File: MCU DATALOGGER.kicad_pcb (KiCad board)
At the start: 2 copper layers, 54.3 x 31.6 mm, 30 parts, among them J1 Conn_01x04_Pin, J2 Conn_01x04_Pin, J3 Conn_01x09_Pin, J4 Conn_02x03_Odd_Even, U1 24LC1025, U2 24LC1025, U4 ATMEGA328P-AU, U5 DS1337S_, Y1 32.768 KHz, Y2 16 MHz

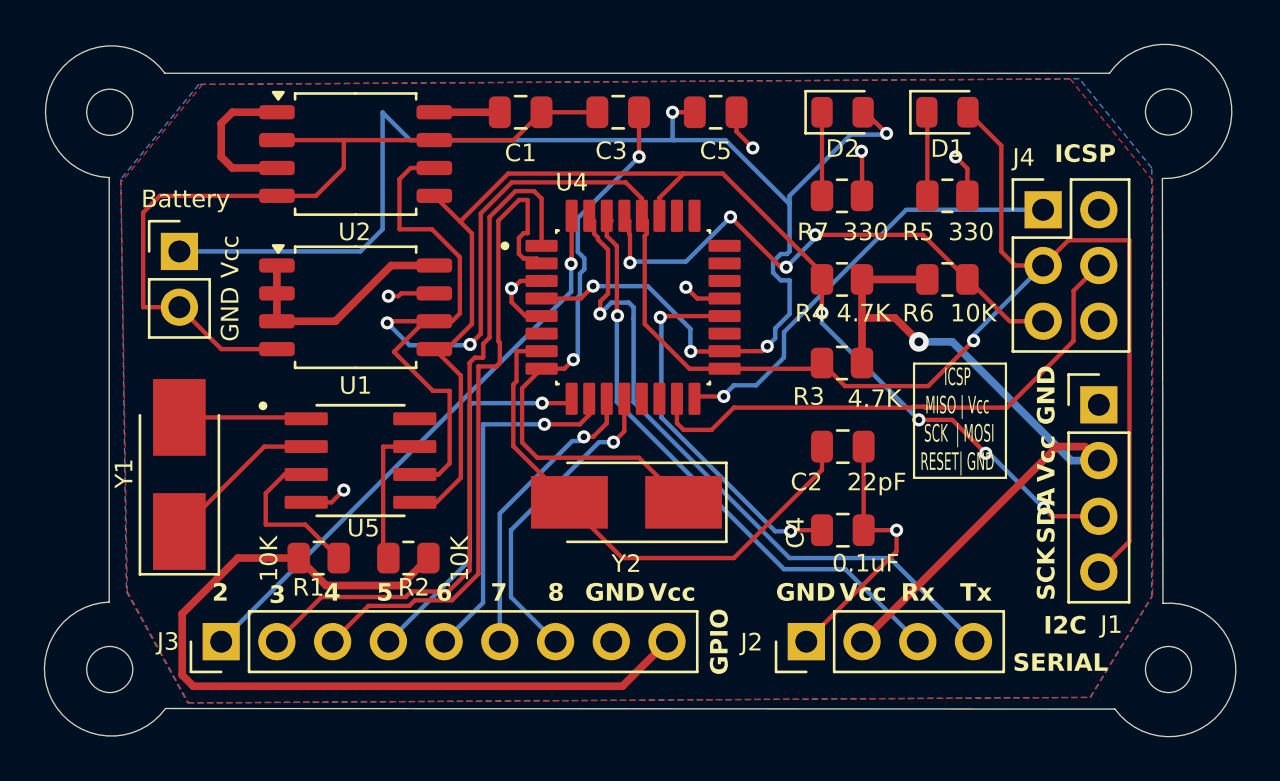
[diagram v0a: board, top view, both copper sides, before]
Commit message: Updated
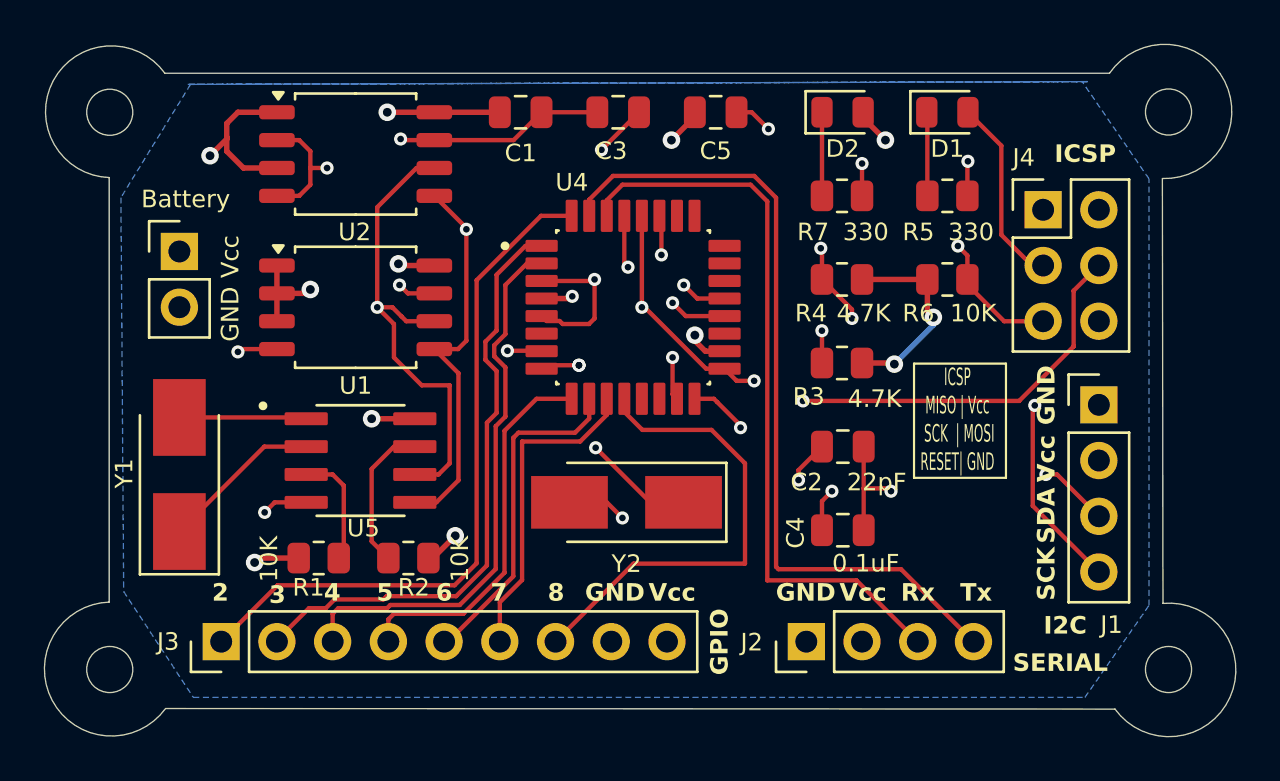
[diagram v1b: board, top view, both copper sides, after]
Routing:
- net /Vcc: track 160.6 -> 46.3 mm, vias 6 -> 13
- net GND: track 65.6 -> 39.9 mm, vias 8 -> 11
- net /SCK: track 99.9 -> 87.7 mm, vias 3 -> 5
- net /D8: track 14.4 -> 21.8 mm, vias 1 -> 0
- net /RX: track 27.4 -> 33.9 mm, vias 1 -> 0
- net /TX: track 31.1 -> 37.3 mm, vias 1 -> 0
- net /D2: track 26.0 -> 31.6 mm, vias 1 -> 0
- net /D4: track 30.6 -> 25.2 mm
- net /D3: track 32.0 -> 27.5 mm
- net Net-(U4-AREF): track 17.0 -> 20.2 mm
- net /SDA: track 57.9 -> 55.0 mm, vias 4 -> 5
- net Net-(U5-~{INTA}): track 7.58 -> 5.32 mm
- net /MISO: track 20.2 -> 22.1 mm
- net Net-(U4-PB7): track 26.6 -> 24.8 mm, vias 2 -> 4
- net /MOSI: track 25.0 -> 26.6 mm, vias 0 -> 2
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- added copper zone on In2.Cu, net /Vcc
- removed copper zone on F.Cu, net /Vcc
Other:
- copper layers 2 -> 4
- board text removed: "0.2000 mm / 0.0000 mm"
- board text removed: "0.3000 mm"
- board text removed: "1.6000 mm"
- board text removed: "54.3109 mm x 31.5621 mm"
- board text removed: "BOARD CHARACTERISTICS"
- board text removed: "Board Thickness:"
- board text removed: "Board overall dimensions:"
- board text removed: "Castellated pads:"
- board text removed: "Copper Finish:"
- board text removed: "Copper Layer Count:"
- board text removed: "Edge card connectors:"
- board text removed: "Impedance Control:"
- board text removed: "Min hole diameter:"
- board text removed: "Min track/spacing:"
- board text removed: "No"
- board text removed: "None"
- board text removed: "Plated Board Edge:"
